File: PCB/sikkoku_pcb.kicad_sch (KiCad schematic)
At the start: 19 parts, among them J1 Conn_01x03, SW1 SW_PUSH, SW10 SW_PUSH, SW11 SW_PUSH, SW12 SW_PUSH, SW13 SW_PUSH, SW14 SW_PUSH, SW15 SW_PUSH, SW16 SW_PUSH, SW17 SW_PUSH, SW2 SW_PUSH, SW3 SW_PUSH, SW4 SW_PUSH, SW5 SW_PUSH, SW6 SW_PUSH, SW7 SW_PUSH, SW8 SW_PUSH, SW9 SW_PUSH

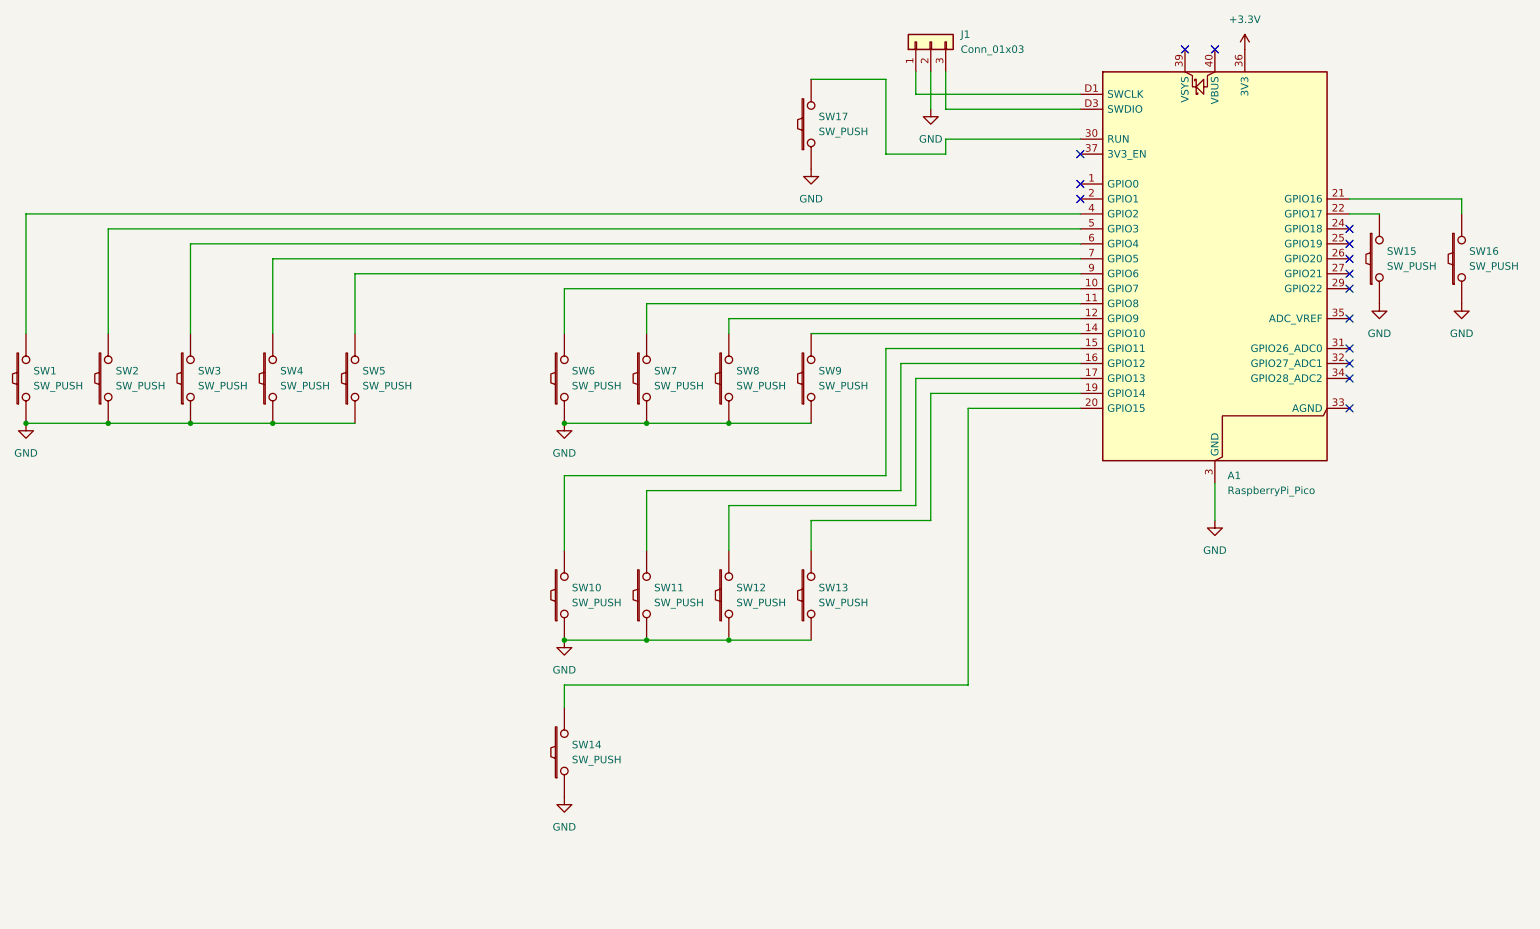
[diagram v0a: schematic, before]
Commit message: 配線が完了 DRC済
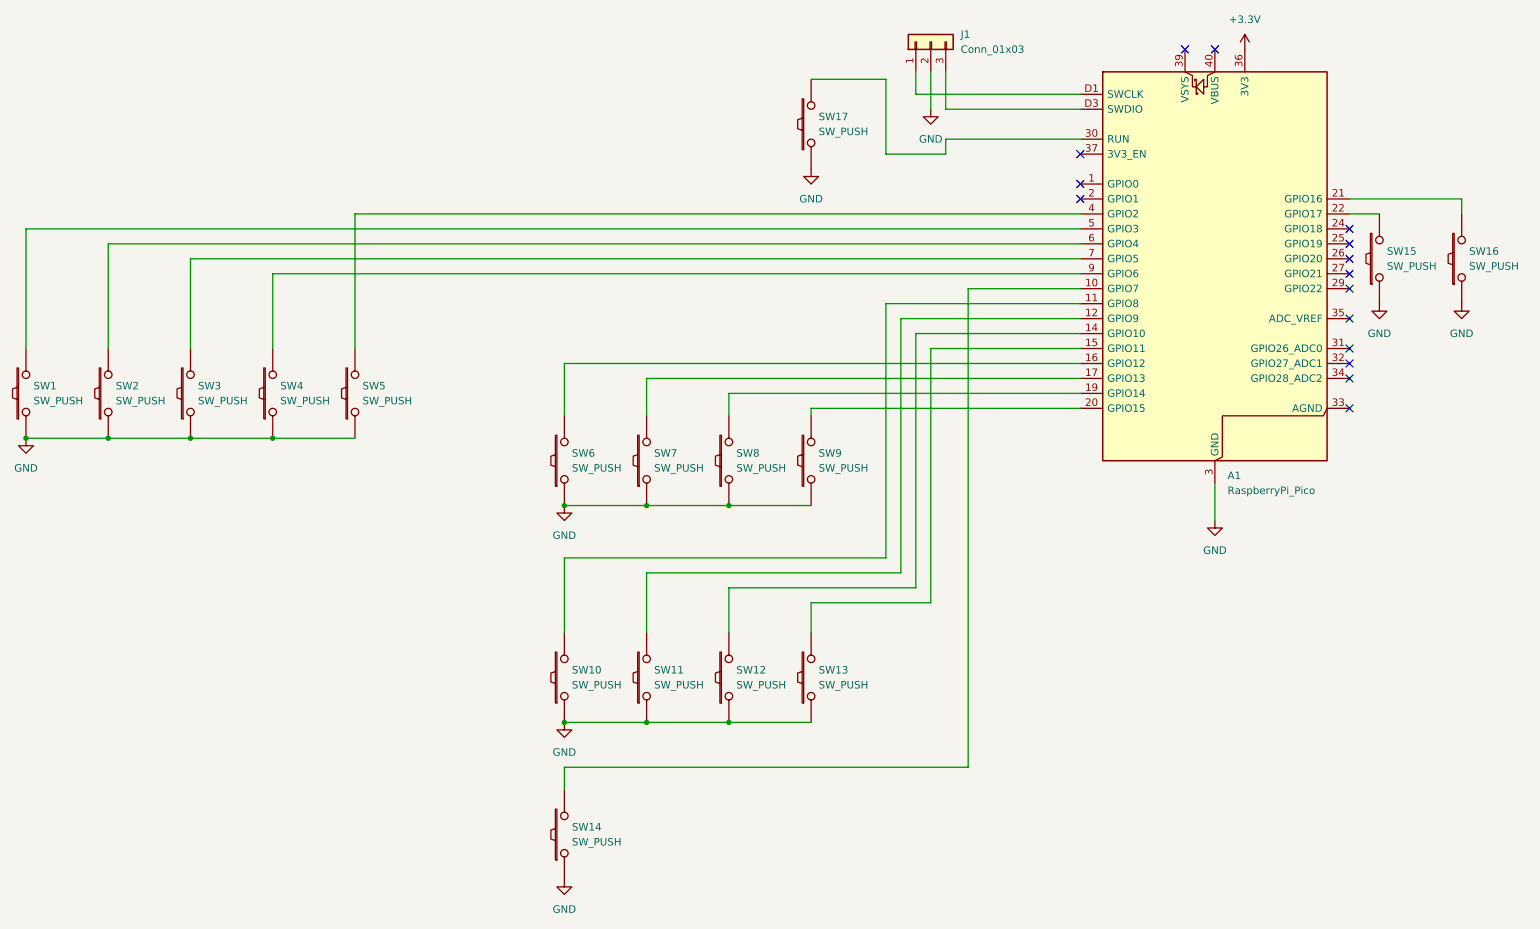
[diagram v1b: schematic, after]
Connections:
- net at A1.10 (GPIO7): now also SW14.2; no longer SW6.2
- net at A1.11 (GPIO8): now also SW10.2; no longer SW7.2
- net at A1.12 (GPIO9): now also SW11.2; no longer SW8.2
- net at A1.14 (GPIO10): now also SW12.2; no longer SW9.2
- net at A1.15 (GPIO11): now also SW13.2; no longer SW10.2
- net at A1.16 (GPIO12): now also SW6.2; no longer SW11.2
- net at A1.17 (GPIO13): now also SW7.2; no longer SW12.2
- net at A1.19 (GPIO14): now also SW8.2; no longer SW13.2
- net at A1.20 (GPIO15): now also SW9.2; no longer SW14.2
- net at A1.4 (GPIO2): now also SW5.2; no longer SW1.2
- net at A1.5 (GPIO3): now also SW1.2; no longer SW2.2
- net at A1.6 (GPIO4): now also SW2.2; no longer SW3.2
- net at A1.7 (GPIO5): now also SW3.2; no longer SW4.2
- net at A1.9 (GPIO6): now also SW4.2; no longer SW5.2
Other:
- moved on the sheet: SW1, SW10, SW11, SW12, SW13, SW14, SW2, SW3, SW4, SW5, SW6, SW7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
